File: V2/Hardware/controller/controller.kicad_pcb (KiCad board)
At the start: 2 copper layers, 45 parts, among them J0 Molex_PSU_F, J2 Flat_7seg_F, J3 Rpi_DATA_F_3.3V, Q0 BD139-16, Q1 BD139-16, Q2 BD139-16, Q3 BD139-16, Q4 BD139-16, Q5 BD139-16, Q6 BD139-16, U1 ATtiny2313-20PU

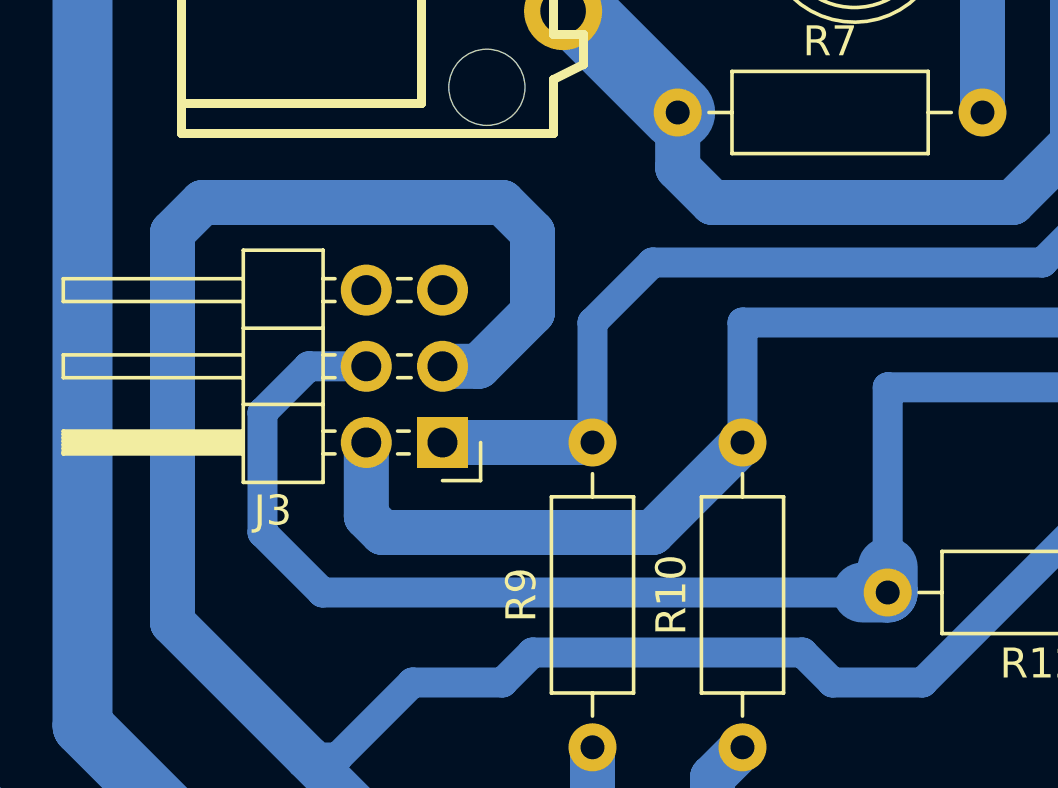
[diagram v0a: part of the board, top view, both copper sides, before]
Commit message: Finish PCBs
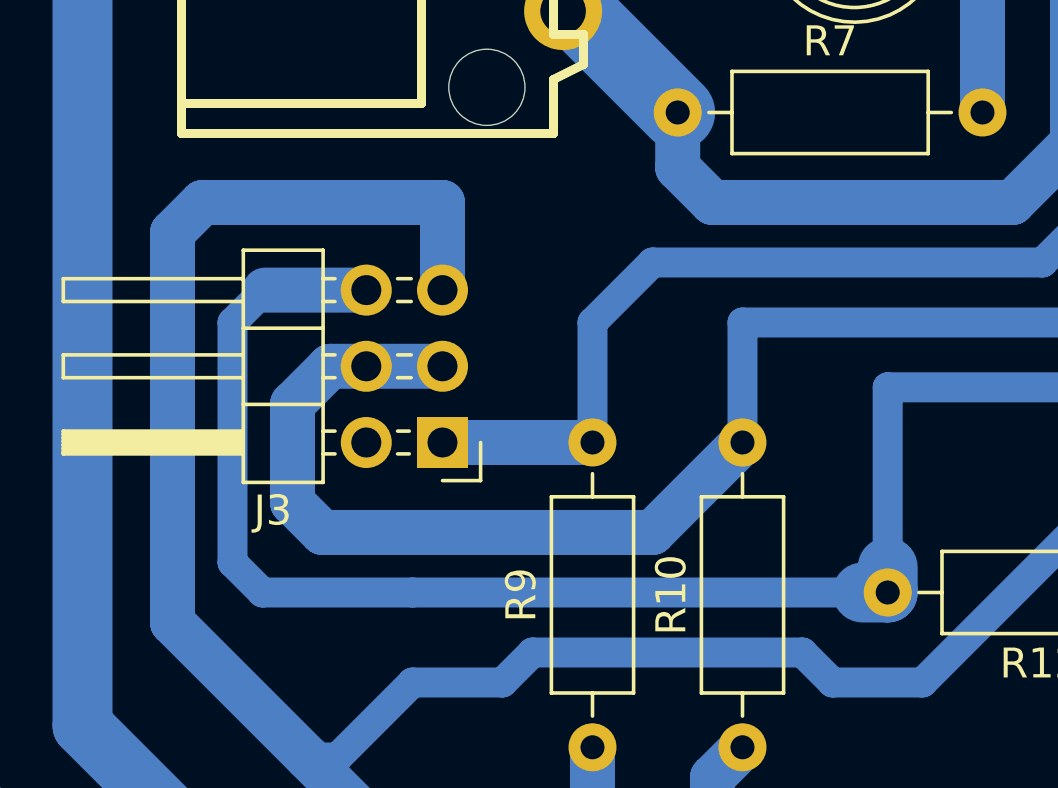
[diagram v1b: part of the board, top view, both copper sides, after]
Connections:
- net /DATA0 renamed /BIT_D
- J3 pad 2: /DATA1 -> Net-(J3-Pad2)
- J3 pad 3: /DATA2 -> /BIT_C
- J3 pad 4: /DATA3 -> /BIT_C
- J3 pad 5: Net-(J3-Pad5) -> /BIT_B
- J3 pad 6: Net-(J3-Pad6) -> /BIT_A
- R10 pad 2: /DATA1 -> /BIT_C
- R11 pad 2: /DATA2 -> /BIT_B
- R12 pad 2: /DATA3 -> /BIT_A
- U1 pad 7: /DATA1 -> /BIT_C
- U1 pad 8: /DATA2 -> /BIT_B
- U1 pad 9: /DATA3 -> /BIT_A
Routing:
- net /DATA2: track 87.7 -> 0.00 mm, vias 2 -> 0
- net /BIT_B: track 0.00 -> 80.8 mm, vias 0 -> 2
- net /BIT_A: track 0.00 -> 57.9 mm
- net /DATA3: track 52.5 -> 0.00 mm
- net /BIT_C: track 0.00 -> 51.4 mm
- net /DATA1: track 42.4 -> 0.00 mm
